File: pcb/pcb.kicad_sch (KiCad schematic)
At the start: 51 parts, among them J1 Ribbon Cable Header, J2 Ribbon Cable Header, J3 ISP, SW1 Cherry MX Grey Switch w/ Gree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, SW2 Cherry MX Grey Switch w/ Gree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, SW3 1241.1100.7095, SW4 SW_SPST, U1 Display Driver, U2 Display Driver, U3 MCU, U4 Inverter, 3 Channels, U5 3:8 Demux, U6 NOR, 4 Channels, U7 OR, 2 Channels, U8 5V Buck Voltage Regulator, Y1 20MHz

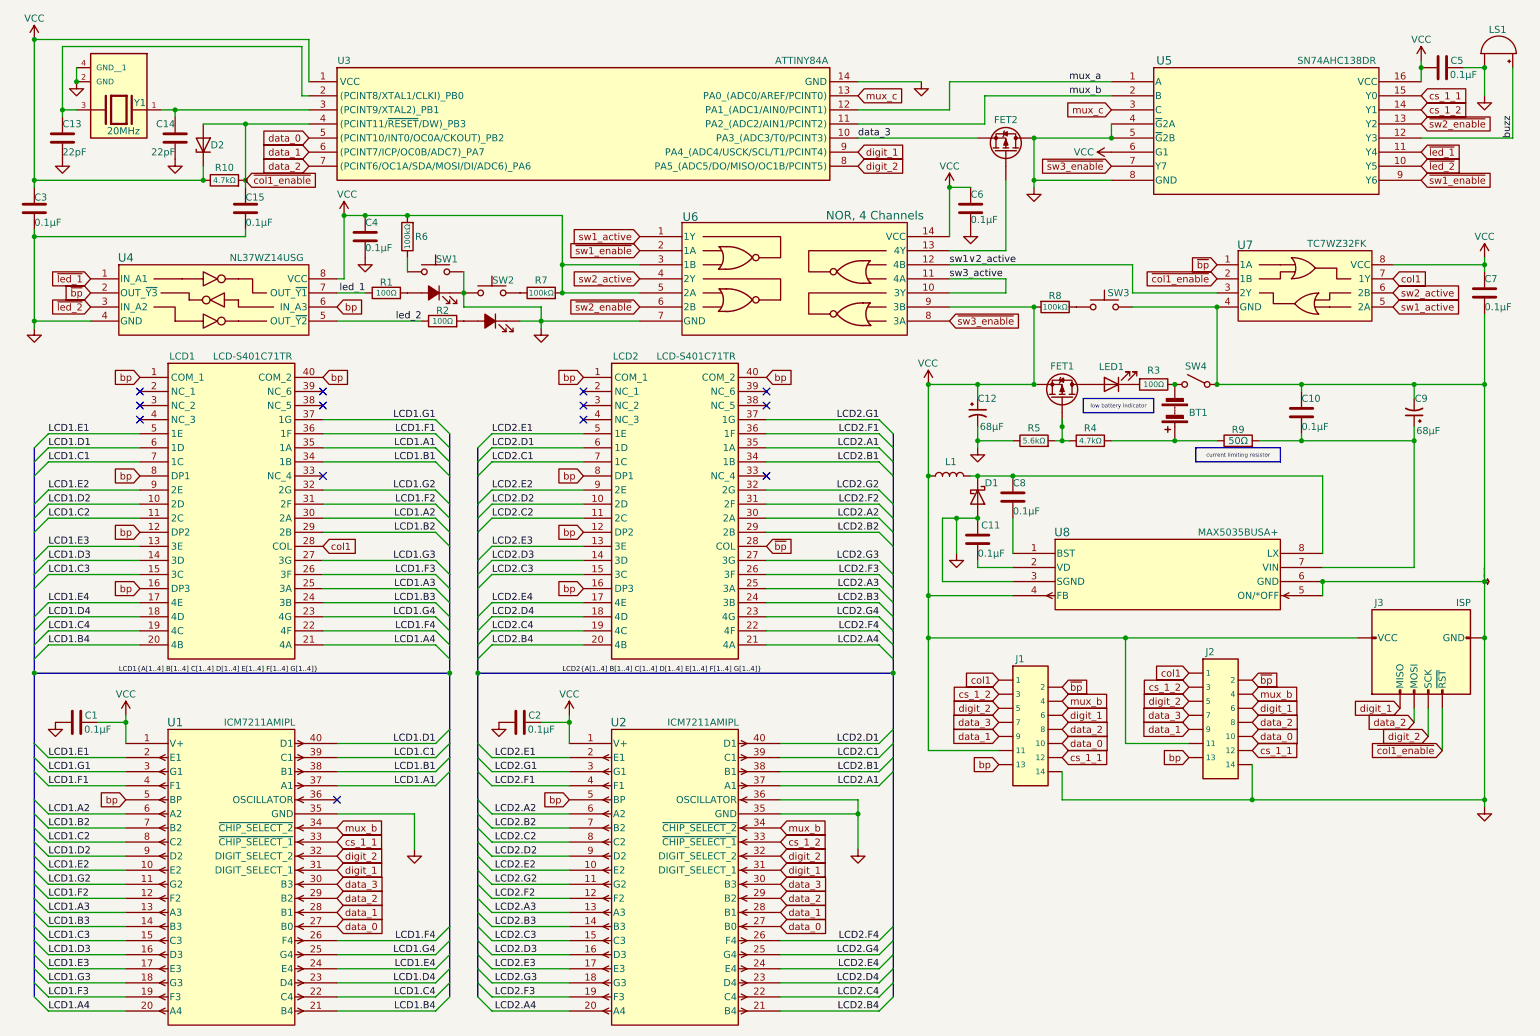
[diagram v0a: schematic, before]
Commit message: crush every error
Signed-off-by: Michael Darr <michael.e.darr@gmail.com>
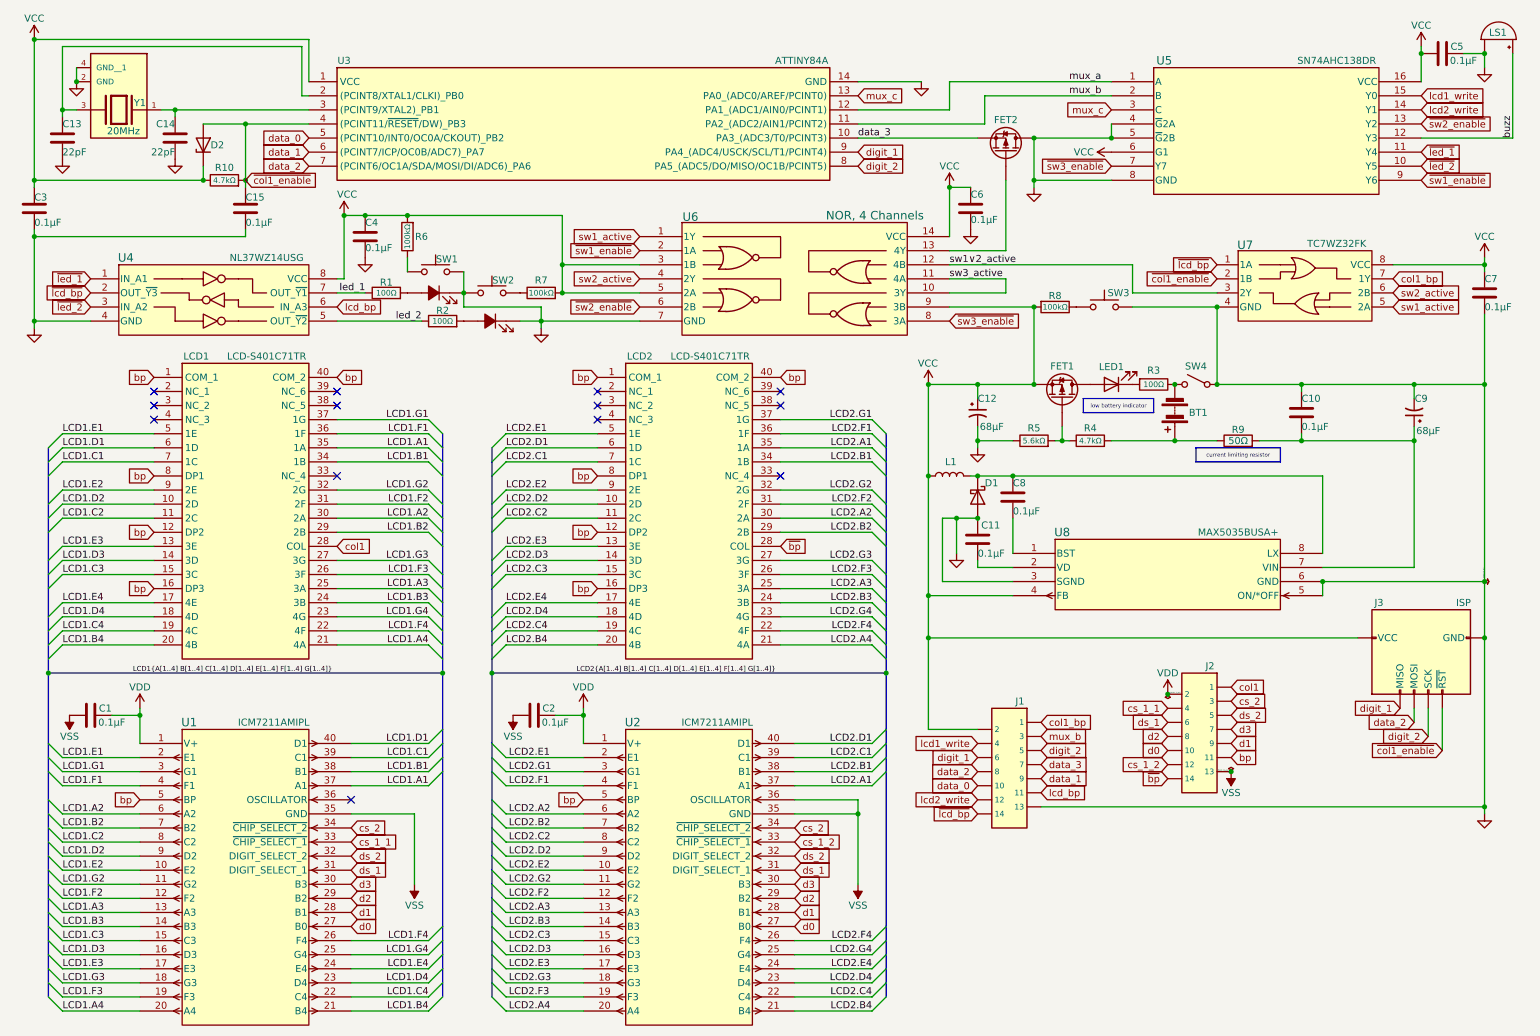
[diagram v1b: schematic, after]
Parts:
- SW1, SW2: value Cherry MX Grey Switch w/ Green LED -> MX Grey w/ LED
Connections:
- net GND: now also J1.13; no longer C1.1, C2.1, J1.14, J2.14, U1.35 (GND), U2.35 (GND), U2.36 (OSCILLATOR)
- net VCC: now also J1.2; no longer C1.2, C2.2, J1.11, J2.11, U1.1 (V+), U2.1 (V+)
- net bp: now also J2.11; no longer J1.13, J2.13, U4.6 (IN_A3)
- net col1: no longer J1.1, U7.7 (1Y)
- net cs_1_1: now also J2.4; no longer J1.12, J2.12, U5.15 (Y0)
- net cs_1_2: now also J2.12; no longer J1.3, J2.3, U5.14 (Y1)
- net data_0: no longer J2.10, U1.27 (B0), U2.27 (B0)
- net data_1: no longer J2.9, U1.28 (B1), U2.28 (B1)
- net data_2: no longer J2.8, U1.29 (B2), U2.29 (B2)
- net data_3: no longer J2.7, U1.30 (B3), U2.30 (B3)
- net digit_1: no longer J2.6, U1.31 (DIGIT_SELECT_1), U2.31 (DIGIT_SELECT_1)
- net digit_2: no longer J2.5, U1.32 (DIGIT_SELECT_2), U2.32 (DIGIT_SELECT_2)
- net mux_b: now also J1.3; no longer J1.4, J2.4, U1.34 (~{CHIP_SELECT_2}), U2.34 (~{CHIP_SELECT_2})
- net ~{bp}: now also J2.14; no longer J1.2, J2.2, U4.2 (OUT_~{Y3}), U7.1 (1A)
- new net VDD: C1.2, C2.2, J2.2, U1.1 (V+), U2.1 (V+)
- new net VSS: C1.1, C2.1, J2.13, U1.35 (GND), U2.35 (GND), U2.36 (OSCILLATOR)
- new net col1_bp: J1.1, U7.7 (1Y)
- new net cs_2: J2.3, U1.34 (~{CHIP_SELECT_2}), U2.34 (~{CHIP_SELECT_2})
- new net d0: J2.10, U1.27 (B0), U2.27 (B0)
- new net d1: J2.9, U1.28 (B1), U2.28 (B1)
- new net d2: J2.8, U1.29 (B2), U2.29 (B2)
- new net d3: J2.7, U1.30 (B3), U2.30 (B3)
- new net ds_1: J2.6, U1.31 (DIGIT_SELECT_1), U2.31 (DIGIT_SELECT_1)
- new net ds_2: J2.5, U1.32 (DIGIT_SELECT_2), U2.32 (DIGIT_SELECT_2)
- new net lcd1_write: J1.4, U5.15 (Y0)
- new net lcd2_write: J1.12, U5.14 (Y1)
- new net lcd_bp: J1.11, U4.6 (IN_A3)
- new net ~{lcd_bp}: J1.14, U4.2 (OUT_~{Y3}), U7.1 (1A)
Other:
- moved on the sheet: C1, C2, C5, J1, J2, LCD1, LCD2, LS1, U1, U2
